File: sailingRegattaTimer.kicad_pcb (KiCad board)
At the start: 2 copper layers, 69.5 x 54.5 mm, 25 parts, among them J1-Red-1M1 Conn_01x02_Socket, J10-12v-In1 Conn_01x02_Socket, J2-Yel-2M1 Conn_01x02_Socket, J3-Grn-3M1 J3-Grn-3M, J4-Blu-5M1 J4-Blu-5M1, J5-5v-LED1 Conn_01x02_Socket, J6-Reset1 J6-Reset, J7-Ext-Buz1 Conn_01x02_Socket, J8-Pololu-VReg1 Conn_01x04_Socket, J9-Relay1 Conn_01x03_Socket

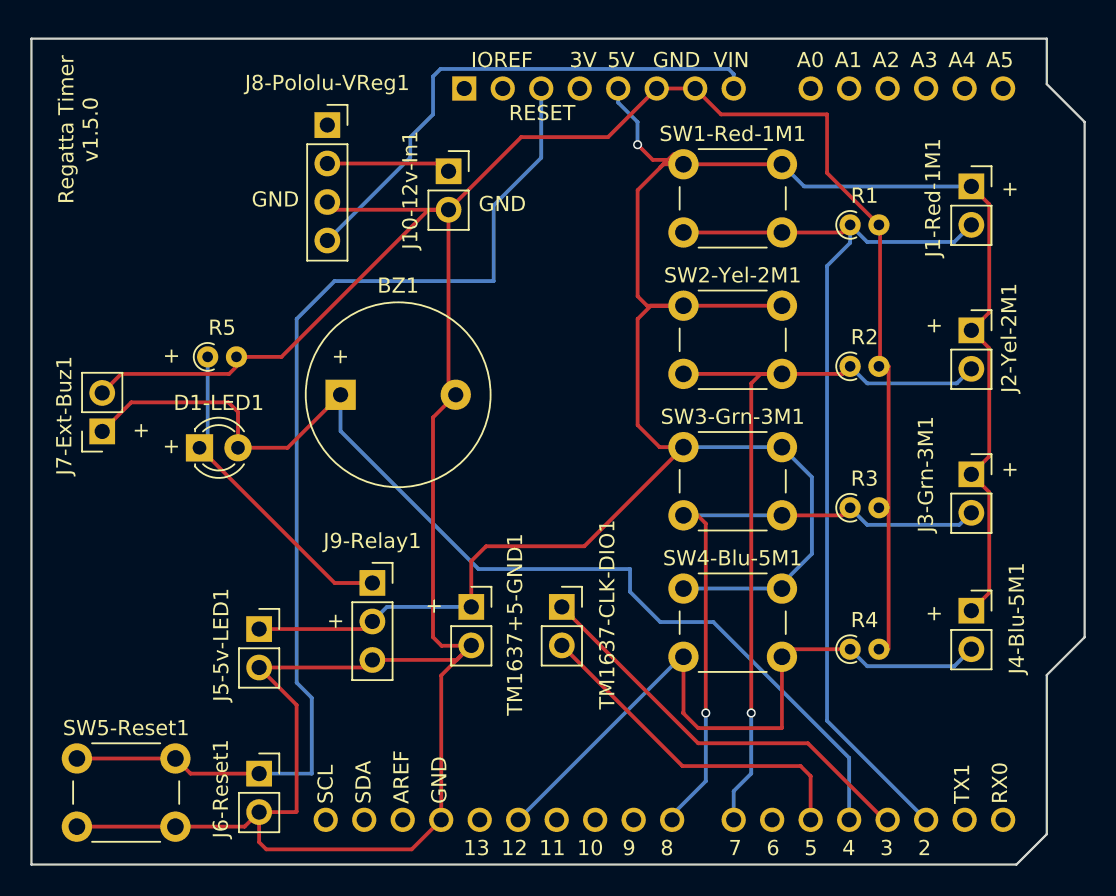
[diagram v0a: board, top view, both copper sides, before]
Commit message: incremental save
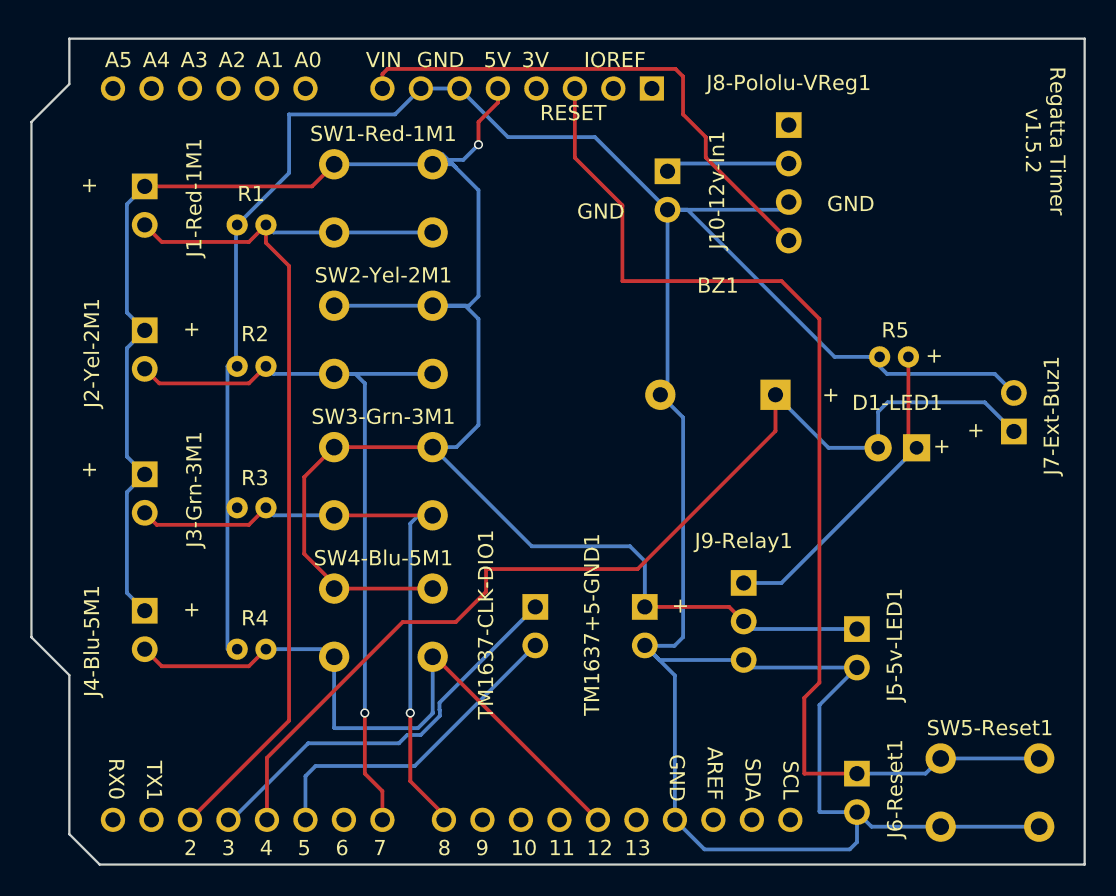
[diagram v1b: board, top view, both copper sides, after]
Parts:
- A1, BZ1, D1-LED1, J1-Red-1M1, J10-12v-In1, J2-Yel-2M1, J3-Grn-3M1, J4-Blu-5M1, J5-5v-LED1, J6-Reset1, J7-Ext-Buz1, J8-Pololu-VReg1, J9-Relay1, R2, R3, R4, R5, SW1-Red-1M1, SW2-Yel-2M1, SW3-Grn-3M1, SW4-Blu-5M1, SW5-Reset1, TM1637+5-GND1, TM1637-CLK-DIO1: moved to B.Cu
- R1: value R -> ${Reference}; moved to B.Cu
- moved SW5-Reset1 63.5 mm to (215.0, 90.5), turned to 180 degrees
- moved J7-Ext-Buz1 60.2 mm to (213.3, 68.9), turned to 0 degrees
- moved J1-Red-1M1 54.6 mm to (156.0, 52.8), turned to 180 degrees
- moved J2-Yel-2M1 54.6 mm to (156.0, 62.2), turned to 180 degrees
- moved J3-Grn-3M1 54.6 mm to (156.0, 71.8), turned to 180 degrees
- moved J4-Blu-5M1 54.6 mm to (156.0, 80.8), turned to 180 degrees
- moved D1-LED1 47.3 mm to (206.9, 70.0), turned to 180 degrees
- moved R5 46.2 mm to (206.4, 64.0), turned to 180 degrees
- moved J5-5v-LED1 39.4 mm to (203.0, 82.0), turned to 180 degrees
- moved J6-Reset1 39.4 mm to (203.0, 91.5), turned to 180 degrees
- moved R1 38.6 mm to (164.0, 55.3), turned to 180 degrees
- moved R2 38.6 mm to (164.0, 64.6), turned to 180 degrees
- moved R3 38.6 mm to (164.0, 74.0), turned to 180 degrees
- moved R4 38.6 mm to (164.0, 83.3), turned to 180 degrees
- moved J8-Pololu-VReg1 30.4 mm to (198.5, 48.7), turned to 180 degrees
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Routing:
- net Net-(A1-D5): track 22.9 -> 21.6 mm
- net Net-(A1-D3): track 27.3 -> 26.6 mm
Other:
- outline, holes or cut-outs redrawn
- board text added: "R1"
- board text added: "Regatta Timer v1.5.2"
- board text removed: "Regatta Timer v1.5.0"
